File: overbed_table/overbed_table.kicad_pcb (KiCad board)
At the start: 2 copper layers, 289 parts, among them CN10 DLL-5569-2AW, CN2 KF2EDGRC-5.08-4P, CN3 KF2EDGRC-5.08-4P, CN4 DLL-5569-6AW, CN5 KF2EDGRC-5.08-4P, CN6 DLL-5569-6AW, CN7 KF2EDGRC-5.08-4P, CN8 DLL-5569-2AW, CN9 DLL-5569-2AW, Q1 BSS138, Q2 BSS138, Q3 BSS138, Q4 AON7524, Q5 AON7524, Q6 AON7524, SW1 KH-6X6X6H-STM, SW10 KH-6X6X6H-STM, SW11 KH-6X6X6H-STM, SW12 KH-6X6X6H-STM, SW13 KH-6X6X6H-STM, SW14 KH-6X6X6H-STM, SW15 KH-6X6X6H-STM, SW16 KH-6X6X6H-STM, SW17 KH-6X6X6H-STM, SW18 KH-6X6X6H-STM, SW2 KH-6X6X6H-STM, SW3 KH-6X6X6H-STM, SW4 KH-6X6X6H-STM, SW5 KH-6X6X6H-STM, SW6 KH-6X6X6H-STM, SW7 KH-6X6X6H-STM, SW8 KH-6X6X6H-STM, SW9 KH-6X6X6H-STM, U1 AP2112K-3.3TRG1, U10 TPS562201DDCR, U11 TPS562201DDCR, U12 TM1638, U13 SS6285M-SO-TP, U14 TMC2209-LA, U15 SP3485EN, U16 SP3485EN, U17 VL53L0CXV0DH1, U18 TPS562201DDCR, U19 PY32F030K28U6TR, U2 ESP32-C3-WROOM-02, U20 WAFER-XH254WZ-2A, U21 WAFER-XH254WZ-2A, U22 WAFER-XH254WZ-4A, U23 KF128-5.08-2P, U24 KF128-5.08-2P, U25 PY32F030K28U6TR, U26 WAFER-XH254WZ-2A, U27 WAFER-XH254WZ-2A, U28 WAFER-XH254WZ-4A, U29 KF128-5.08-2P, U3 WAFER-XH254WZ-2A, U30 KF128-5.08-2P, U31 TMC2209-LA, U32 VL53L0CXV0DH1, U33 TPS562201DDCR, U34 SS6285M-SO-TP, U35 SP3485EN, U4 BSMD2920-500-24V, U5 BSMD2920-500-24V, U6 BSMD2920-500-24V, U7 KF7620-7.62-2P, X1 AFA01-S05FCA-00, X2 AFA01-S05FCA-00, X3 AFA01-S05FCA-00, X4 AFA01-S05FCA-00, X5 AFA01-S05FCA-00, X6 AFA01-S05FCA-00

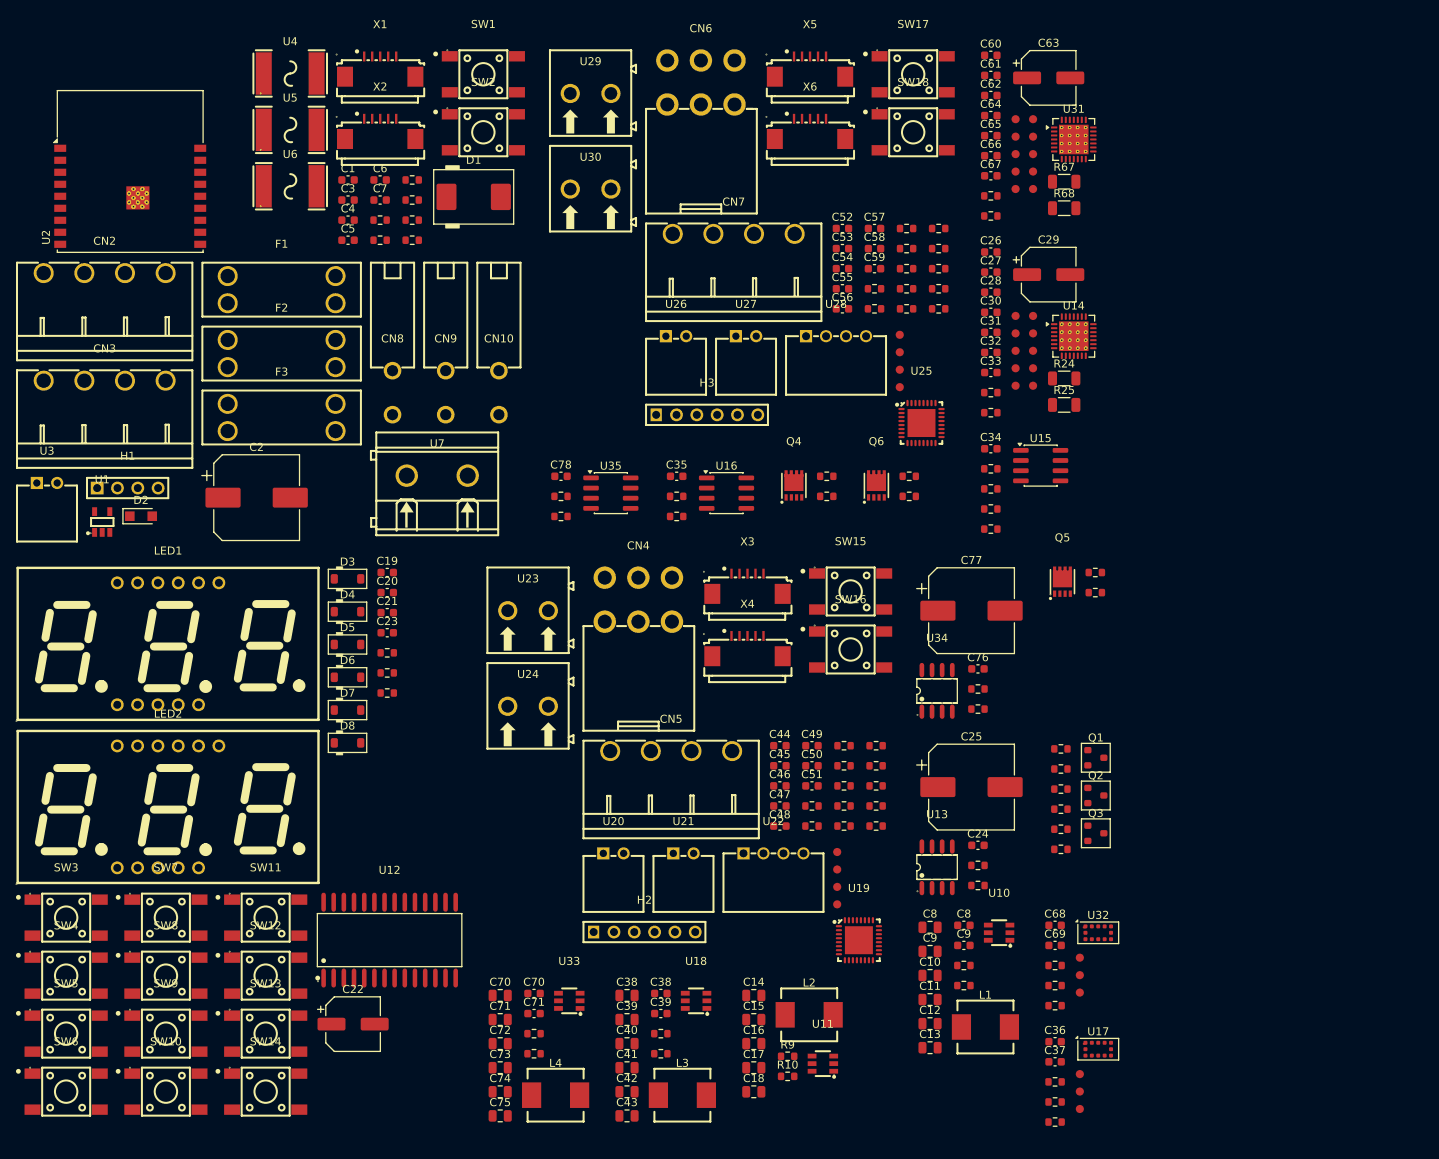
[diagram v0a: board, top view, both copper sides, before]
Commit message: 更新原理图
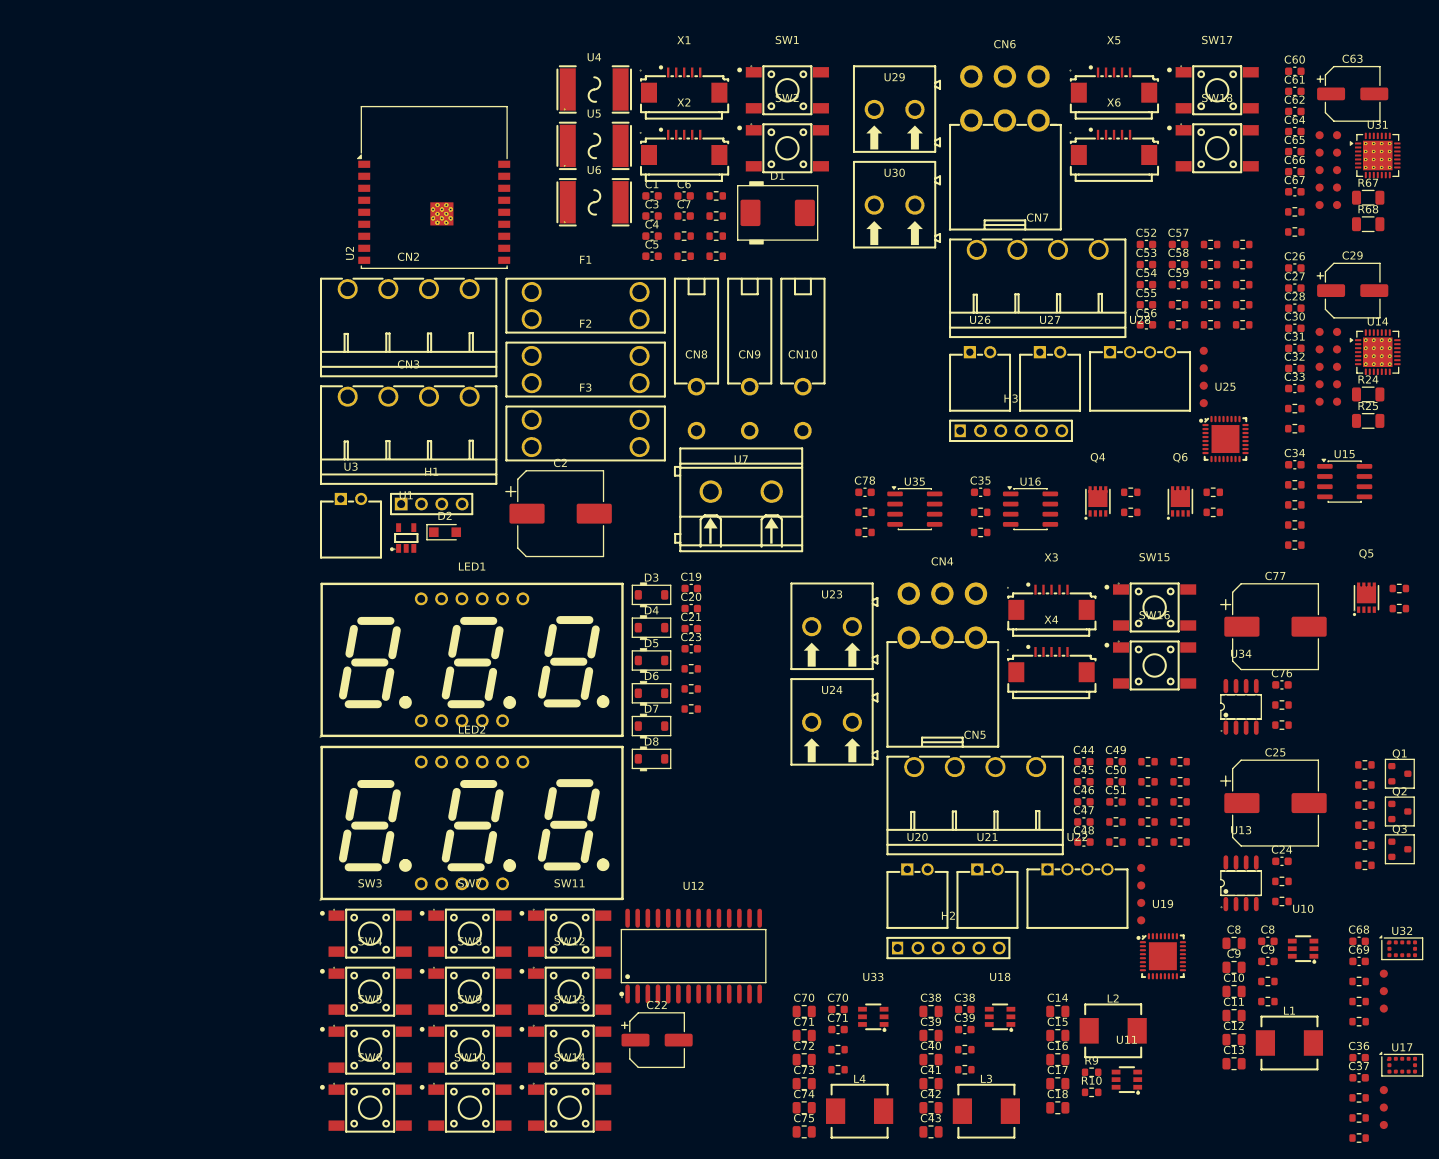
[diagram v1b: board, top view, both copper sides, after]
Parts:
- removed the C38 at (128.4, 155.8)
- removed the C38 at (132.6, 155.5)
- removed the C39 at (132.6, 158.0)
- removed the C39 at (128.4, 158.8)
- removed the C70 at (116.8, 155.5)
- removed the C70 at (112.5, 155.8)
- removed the C71 at (116.8, 158.0)
- removed the C71 at (112.5, 158.8)
- removed the C8 at (166.3, 147.3)
- removed the C8 at (170.5, 147.0)
- removed the C9 at (170.5, 149.5)
- removed the C9 at (166.3, 150.3)
- added C38: 10uF, Capacitor_SMD:C_0603_1608Metric, F.Cu at (170.6, 157.5)
- added C38: 10uF, Capacitor_SMD:C_0805_2012Metric, F.Cu at (166.4, 157.8)
- added C39: 10uF, Capacitor_SMD:C_0805_2012Metric, F.Cu at (166.4, 160.8)
- added C39: 10uF, Capacitor_SMD:C_0603_1608Metric, F.Cu at (170.6, 160.0)
- added C70: 10uF, Capacitor_SMD:C_0603_1608Metric, F.Cu at (154.8, 157.5)
- added C70: 10uF, Capacitor_SMD:C_0805_2012Metric, F.Cu at (150.5, 157.8)
- added C71: 10uF, Capacitor_SMD:C_0603_1608Metric, F.Cu at (154.8, 160.0)
- added C71: 10uF, Capacitor_SMD:C_0805_2012Metric, F.Cu at (150.5, 160.8)
- added C8: 10uF, Capacitor_SMD:C_0603_1608Metric, F.Cu at (208.5, 149.0)
- added C8: 10uF, Capacitor_SMD:C_0805_2012Metric, F.Cu at (204.3, 149.3)
- added C9: 10uF, Capacitor_SMD:C_0805_2012Metric, F.Cu at (204.3, 152.3)
- added C9: 10uF, Capacitor_SMD:C_0603_1608Metric, F.Cu at (208.5, 151.5)
- moved CN10 38.1 mm to (150.4, 82.4)
- moved D1 38.1 mm to (147.2, 58.0)
- moved U1 38.1 mm to (100.8, 98.6)
- moved C1 38.1 mm to (131.5, 55.8)
- moved C10 38.1 mm to (204.3, 155.3)
- moved C11 38.1 mm to (204.3, 158.3)
- moved C12 38.1 mm to (204.3, 161.3)
- moved C13 38.1 mm to (204.3, 164.3)
- moved C14 38.1 mm to (182.2, 157.8)
- moved C15 38.1 mm to (182.2, 160.8)
- moved C16 38.1 mm to (182.2, 163.8)
- moved C17 38.1 mm to (182.2, 166.8)
- moved C18 38.1 mm to (182.2, 169.8)
- moved C19 38.1 mm to (136.4, 104.9)
- moved C2 38.1 mm to (120.1, 95.5)
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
